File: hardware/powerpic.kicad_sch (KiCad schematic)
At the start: 21 parts

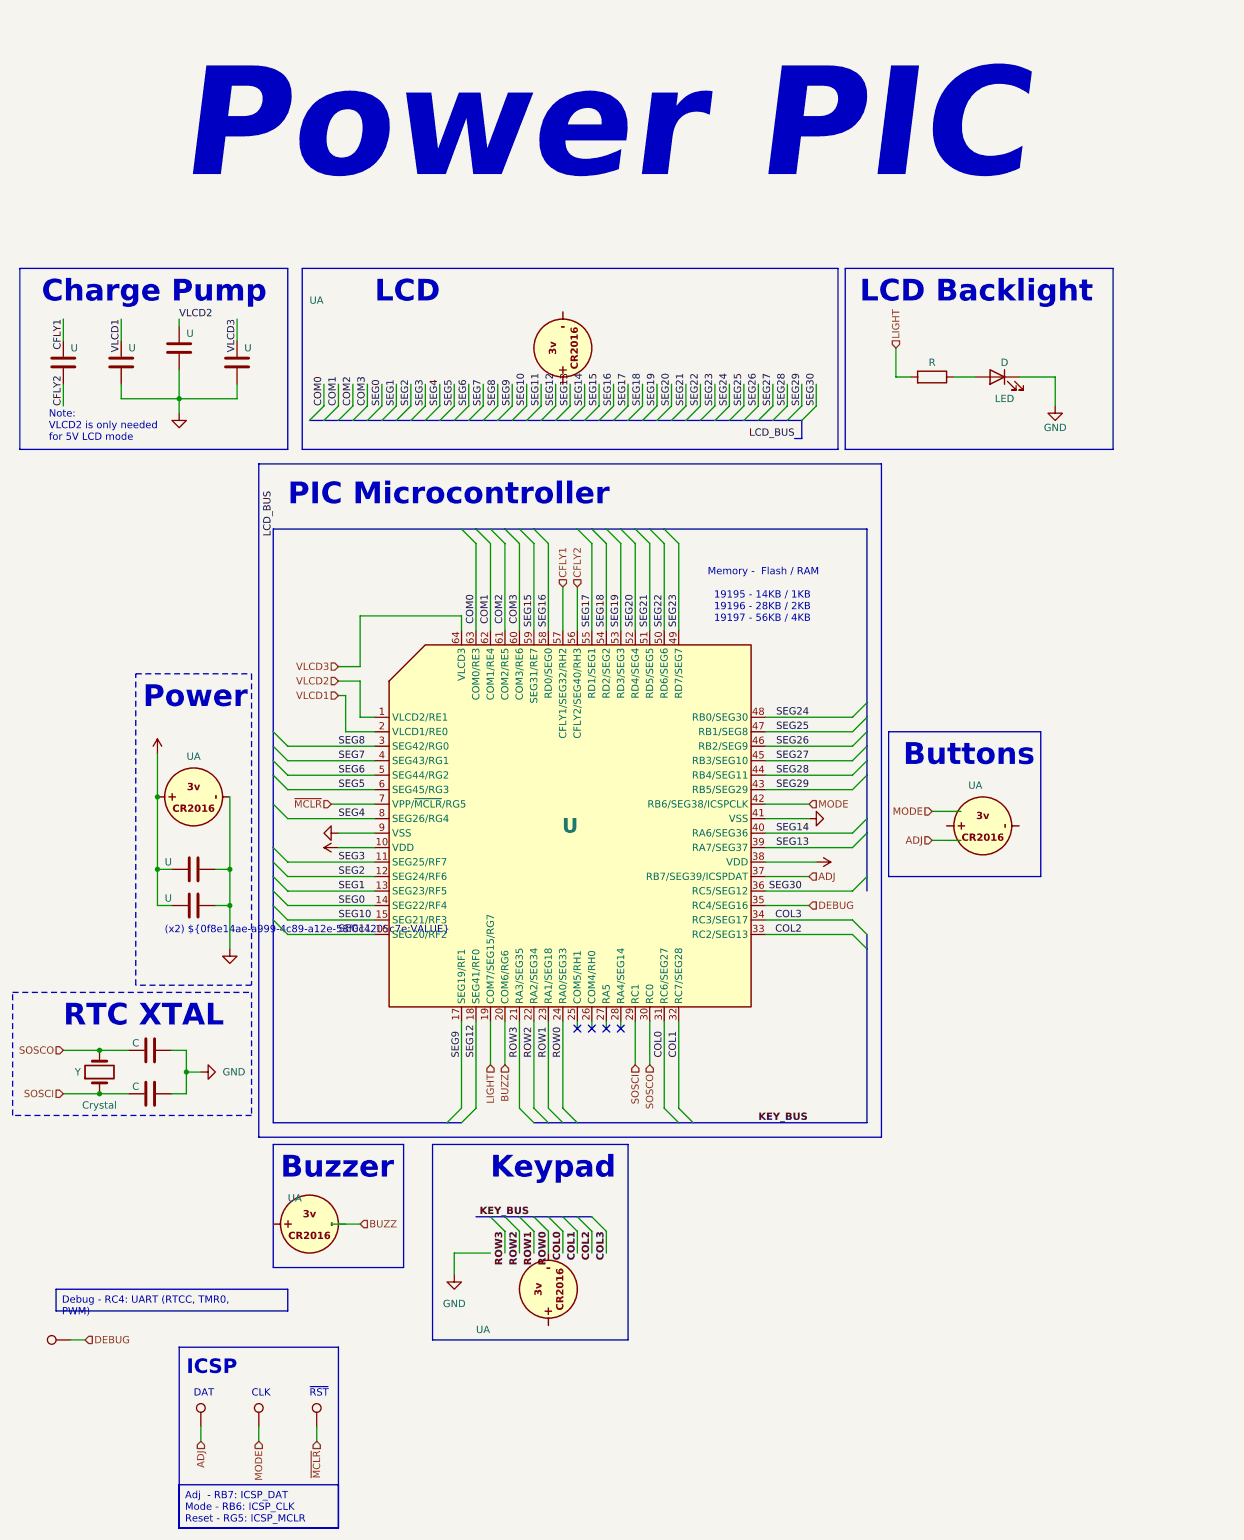
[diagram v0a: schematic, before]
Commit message: Starting work on version 3 of the hardware.
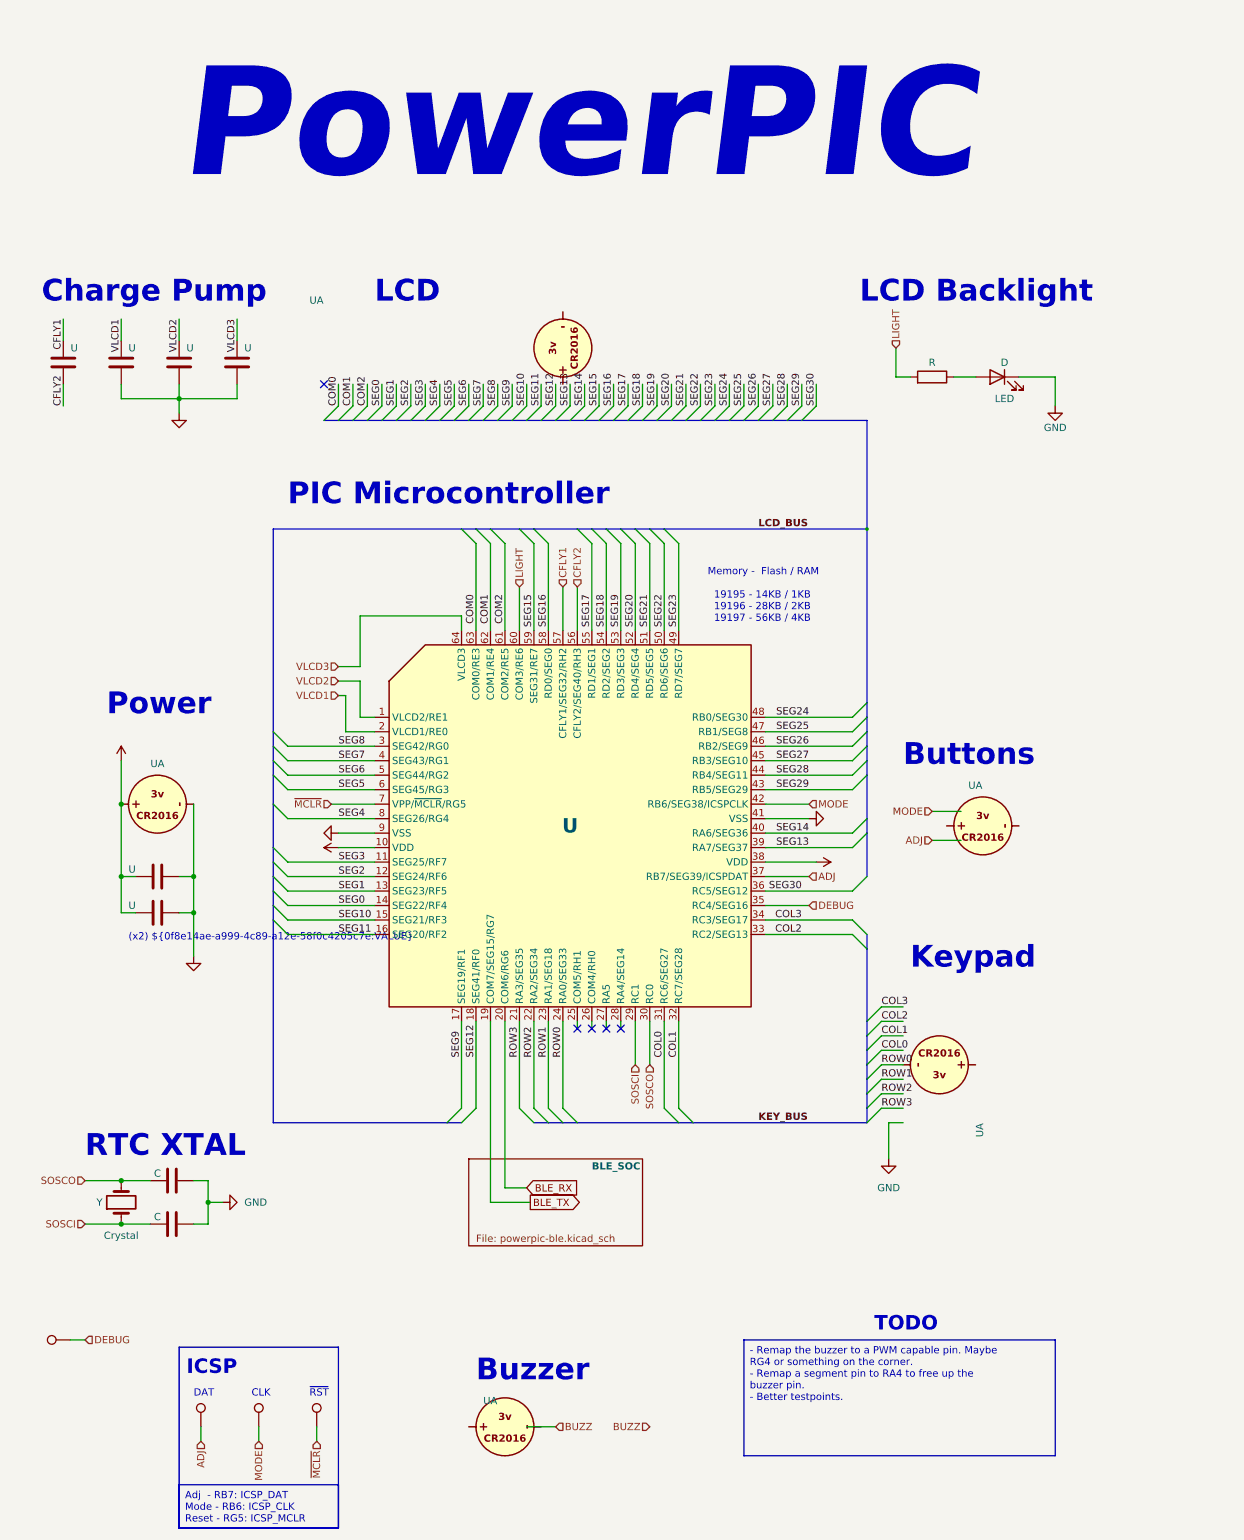
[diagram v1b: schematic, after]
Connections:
- net COM3 is gone; now on net LIGHT: U.60 (COM3/RE6)
- net BUZZ: no longer U.20 (COM6/RG6)
- net LIGHT: no longer U.19 (COM7/SEG15/RG7)
- new net BLE_RX: U.20 (COM6/RG6)
- new net BLE_TX: U.19 (COM7/SEG15/RG7)
- no-connect marks 4 -> 5
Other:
- added sheet BLE_SOC (powerpic-ble.kicad_sch)
- note added: "PowerPIC"
- note added: "TODO"
- note removed: "Note: VLCD2 is only needed for 5V LCD mode"
- note removed: "Power PIC"
- moved on the sheet: C, U, UA, Y
